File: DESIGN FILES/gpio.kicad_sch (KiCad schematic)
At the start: 12 parts, among them U1 MIMXRT1064CVL5B

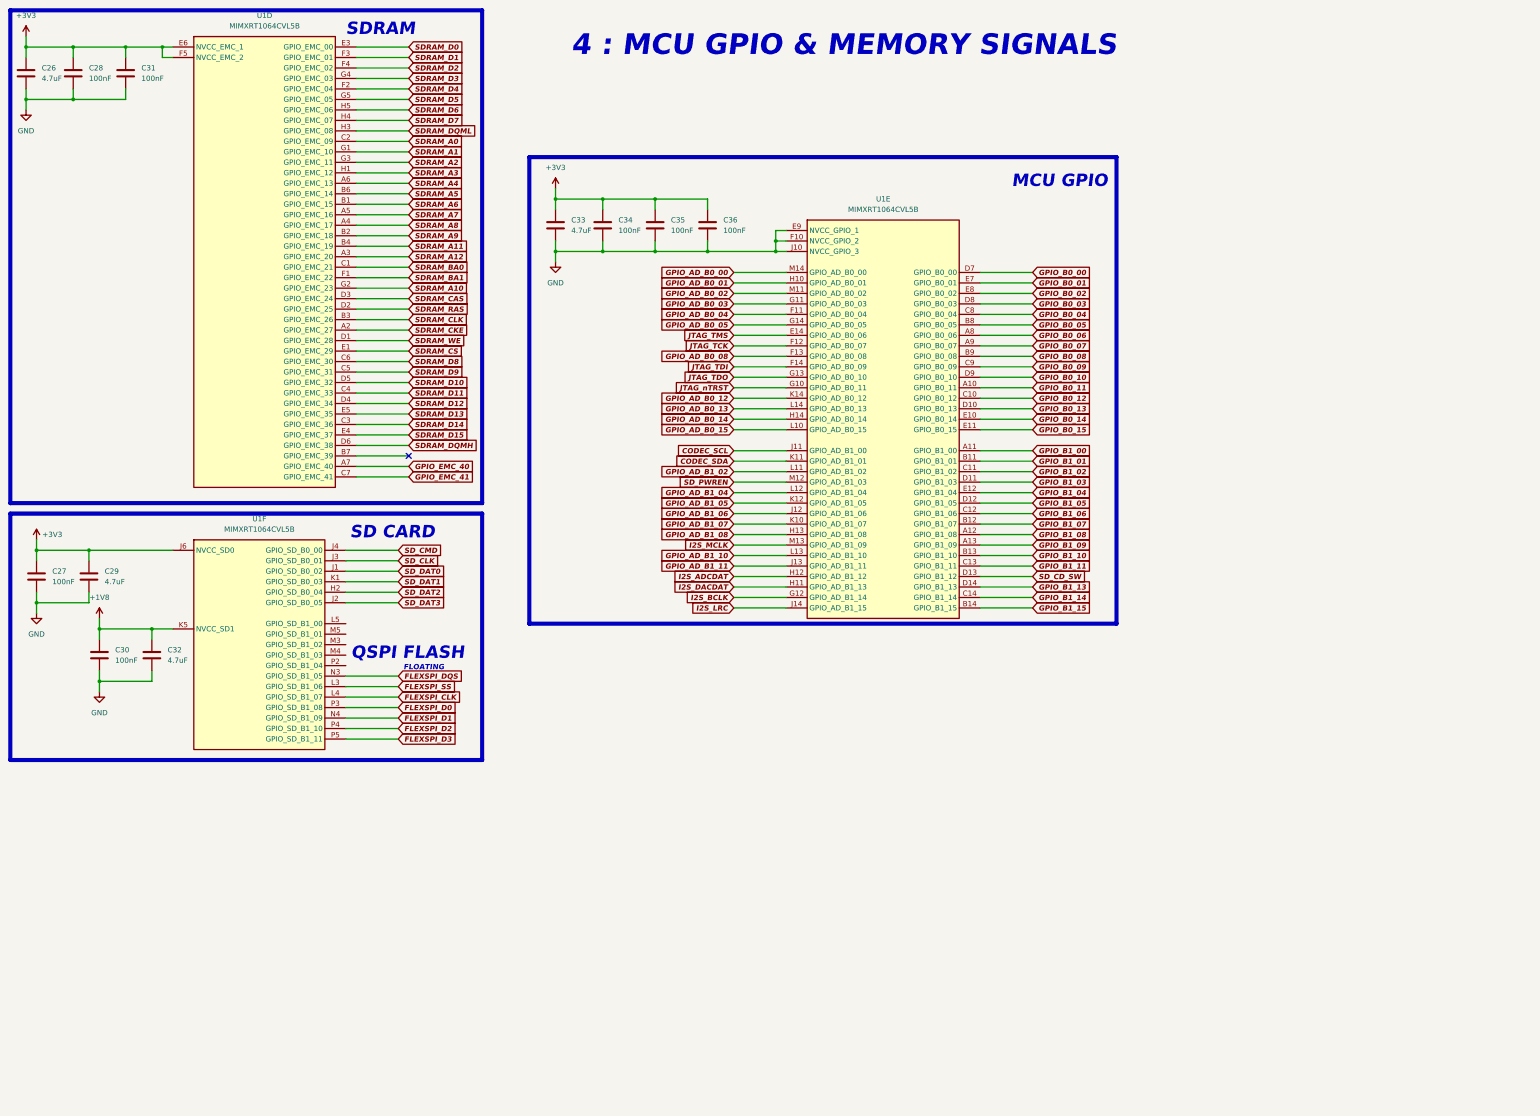
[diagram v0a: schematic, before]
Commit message: schematic edit
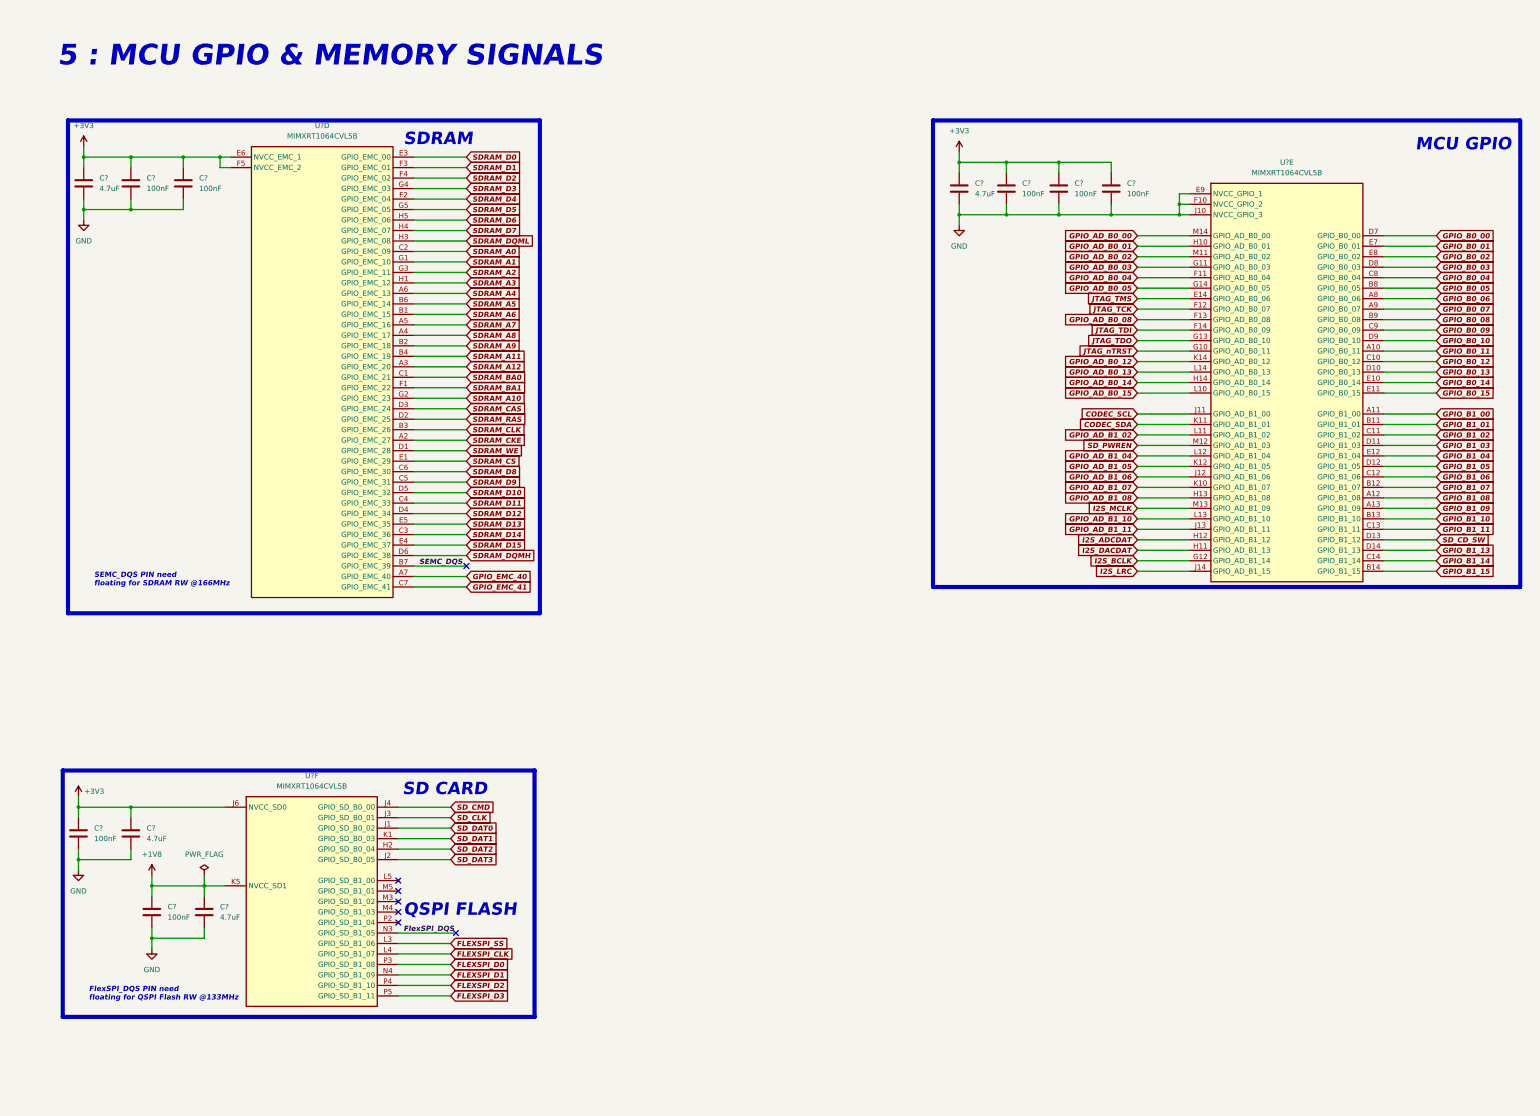
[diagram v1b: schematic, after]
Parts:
- removed C26, C29, C32, C33: 4.7uF, MIMXRT1064 MCU Module:0402_CL05A475MP5NRNC, symbol MIMXRT1064 MCU Module:CL05A475MP5NRNC
- removed C27, C28, C30, C31, C34, C35, C36: 100nF, MIMXRT1064 MCU Module:0402_CL05B104KB54PNC, symbol MIMXRT1064 MCU Module:CL05B104KB54PNC
- removed U1: MIMXRT1064CVL5B, MIMXRT1064 MCU Module:MIMXRT1064CVL5B, symbol MIMXRT1064 MCU Module:MIMXRT1064CVL5B
- added C? (x4): 4.7uF, MIMXRT1064 MCU Module:0402_CL05A475MP5NRNC, symbol MIMXRT1064 MCU Module:CL05A475MP5NRNC
- added C? (x7): 100nF, MIMXRT1064 MCU Module:0402_CL05B104KB54PNC, symbol MIMXRT1064 MCU Module:CL05B104KB54PNC
- added U? (x3): MIMXRT1064CVL5B, MIMXRT1064 MCU Module:MIMXRT1064CVL5B, symbol MIMXRT1064 MCU Module:MIMXRT1064CVL5B
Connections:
- net +1V8: now also C?.1, C?.1, U?.K5 (NVCC_SD1)
- net +3V3: now also C?.1, C?.1, C?.1, C?.1, C?.1, C?.1, C?.1, C?.1, C?.1, U?.E6 (NVCC_EMC_1), U?.F5 (NVCC_EMC_2), U?.J6 (NVCC_SD0)
- net CODEC_SCL: now also U?.J11 (GPIO_AD_B1_00)
- net CODEC_SDA: now also U?.K11 (GPIO_AD_B1_01)
- net FLEXSPI_CLK: now also U?.L4 (GPIO_SD_B1_07)
- net FLEXSPI_D0: now also U?.P3 (GPIO_SD_B1_08)
- net FLEXSPI_D1: now also U?.N4 (GPIO_SD_B1_09)
- net FLEXSPI_D2: now also U?.P4 (GPIO_SD_B1_10)
- net FLEXSPI_D3: now also U?.P5 (GPIO_SD_B1_11)
- net FLEXSPI_SS: now also U?.L3 (GPIO_SD_B1_06)
- net GND: now also C?.2, C?.2, C?.2, C?.2, C?.2, C?.2, C?.2, C?.2, C?.2, C?.2, C?.2, U?.E9 (NVCC_GPIO_1), U?.F10 (NVCC_GPIO_2), U?.J10 (NVCC_GPIO_3)
- net GPIO_AD_B0_00: now also U?.M14 (GPIO_AD_B0_00)
- net GPIO_AD_B0_01: now also U?.H10 (GPIO_AD_B0_01)
- net GPIO_AD_B0_02: now also U?.M11 (GPIO_AD_B0_02)
- net GPIO_AD_B0_03: now also U?.G11 (GPIO_AD_B0_03)
- net GPIO_AD_B0_04: now also U?.F11 (GPIO_AD_B0_04)
- net GPIO_AD_B0_05: now also U?.G14 (GPIO_AD_B0_05)
- net GPIO_AD_B0_08: now also U?.F13 (GPIO_AD_B0_08)
- net GPIO_AD_B0_12: now also U?.K14 (GPIO_AD_B0_12)
- net GPIO_AD_B0_13: now also U?.L14 (GPIO_AD_B0_13)
- net GPIO_AD_B0_14: now also U?.H14 (GPIO_AD_B0_14)
- net GPIO_AD_B0_15: now also U?.L10 (GPIO_AD_B0_15)
- net GPIO_AD_B1_02: now also U?.L11 (GPIO_AD_B1_02)
- net GPIO_AD_B1_04: now also U?.L12 (GPIO_AD_B1_04)
- net GPIO_AD_B1_05: now also U?.K12 (GPIO_AD_B1_05)
- net GPIO_AD_B1_06: now also U?.J12 (GPIO_AD_B1_06)
- net GPIO_AD_B1_07: now also U?.K10 (GPIO_AD_B1_07)
- net GPIO_AD_B1_08: now also U?.H13 (GPIO_AD_B1_08)
- net GPIO_AD_B1_10: now also U?.L13 (GPIO_AD_B1_10)
- net GPIO_AD_B1_11: now also U?.J13 (GPIO_AD_B1_11)
- net GPIO_B0_00: now also U?.D7 (GPIO_B0_00)
- net GPIO_B0_01: now also U?.E7 (GPIO_B0_01)
- net GPIO_B0_02: now also U?.E8 (GPIO_B0_02)
- net GPIO_B0_03: now also U?.D8 (GPIO_B0_03)
- net GPIO_B0_04: now also U?.C8 (GPIO_B0_04)
- net GPIO_B0_05: now also U?.B8 (GPIO_B0_05)
- net GPIO_B0_06: now also U?.A8 (GPIO_B0_06)
- net GPIO_B0_07: now also U?.A9 (GPIO_B0_07)
- net GPIO_B0_08: now also U?.B9 (GPIO_B0_08)
- net GPIO_B0_09: now also U?.C9 (GPIO_B0_09)
- net GPIO_B0_10: now also U?.D9 (GPIO_B0_10)
- net GPIO_B0_11: now also U?.A10 (GPIO_B0_11)
- net GPIO_B0_12: now also U?.C10 (GPIO_B0_12)
- net GPIO_B0_13: now also U?.D10 (GPIO_B0_13)
- net GPIO_B0_14: now also U?.E10 (GPIO_B0_14)
- net GPIO_B0_15: now also U?.E11 (GPIO_B0_15)
- net GPIO_B1_00: now also U?.A11 (GPIO_B1_00)
- net GPIO_B1_01: now also U?.B11 (GPIO_B1_01)
- net GPIO_B1_02: now also U?.C11 (GPIO_B1_02)
- net GPIO_B1_03: now also U?.D11 (GPIO_B1_03)
- net GPIO_B1_04: now also U?.E12 (GPIO_B1_04)
- net GPIO_B1_05: now also U?.D12 (GPIO_B1_05)
- net GPIO_B1_06: now also U?.C12 (GPIO_B1_06)
- net GPIO_B1_07: now also U?.B12 (GPIO_B1_07)
- net GPIO_B1_08: now also U?.A12 (GPIO_B1_08)
- net GPIO_B1_09: now also U?.A13 (GPIO_B1_09)
- net GPIO_B1_10: now also U?.B13 (GPIO_B1_10)
- net GPIO_B1_11: now also U?.C13 (GPIO_B1_11)
- net GPIO_B1_13: now also U?.D14 (GPIO_B1_13)
- net GPIO_B1_14: now also U?.C14 (GPIO_B1_14)
- net GPIO_B1_15: now also U?.B14 (GPIO_B1_15)
- net GPIO_EMC_40: now also U?.A7 (GPIO_EMC_40)
- net GPIO_EMC_41: now also U?.C7 (GPIO_EMC_41)
- net I2S_ADCDAT: now also U?.H12 (GPIO_AD_B1_12)
- net I2S_BCLK: now also U?.G12 (GPIO_AD_B1_14)
- net I2S_DACDAT: now also U?.H11 (GPIO_AD_B1_13)
- net I2S_LRC: now also U?.J14 (GPIO_AD_B1_15)
- net I2S_MCLK: now also U?.M13 (GPIO_AD_B1_09)
- net JTAG_TCK: now also U?.F12 (GPIO_AD_B0_07)
- net JTAG_TDI: now also U?.F14 (GPIO_AD_B0_09)
- net JTAG_TDO: now also U?.G13 (GPIO_AD_B0_10)
- net JTAG_TMS: now also U?.E14 (GPIO_AD_B0_06)
- net JTAG_nTRST: now also U?.G10 (GPIO_AD_B0_11)
- net SDRAM_A0: now also U?.C2 (GPIO_EMC_09)
- net SDRAM_A1: now also U?.G1 (GPIO_EMC_10)
- net SDRAM_A10: now also U?.G2 (GPIO_EMC_23)
- net SDRAM_A11: now also U?.B4 (GPIO_EMC_19)
- net SDRAM_A12: now also U?.A3 (GPIO_EMC_20)
- net SDRAM_A2: now also U?.G3 (GPIO_EMC_11)
- net SDRAM_A3: now also U?.H1 (GPIO_EMC_12)
- net SDRAM_A4: now also U?.A6 (GPIO_EMC_13)
- net SDRAM_A5: now also U?.B6 (GPIO_EMC_14)
- net SDRAM_A6: now also U?.B1 (GPIO_EMC_15)
- net SDRAM_A7: now also U?.A5 (GPIO_EMC_16)
- net SDRAM_A8: now also U?.A4 (GPIO_EMC_17)
- net SDRAM_A9: now also U?.B2 (GPIO_EMC_18)
- net SDRAM_BA0: now also U?.C1 (GPIO_EMC_21)
- net SDRAM_BA1: now also U?.F1 (GPIO_EMC_22)
- net SDRAM_CAS: now also U?.D3 (GPIO_EMC_24)
- net SDRAM_CKE: now also U?.A2 (GPIO_EMC_27)
- net SDRAM_CLK: now also U?.B3 (GPIO_EMC_26)
- net SDRAM_CS: now also U?.E1 (GPIO_EMC_29)
- net SDRAM_D0: now also U?.E3 (GPIO_EMC_00)
- net SDRAM_D1: now also U?.F3 (GPIO_EMC_01)
- net SDRAM_D10: now also U?.D5 (GPIO_EMC_32)
- net SDRAM_D11: now also U?.C4 (GPIO_EMC_33)
- net SDRAM_D12: now also U?.D4 (GPIO_EMC_34)
- net SDRAM_D13: now also U?.E5 (GPIO_EMC_35)
- net SDRAM_D14: now also U?.C3 (GPIO_EMC_36)
- net SDRAM_D15: now also U?.E4 (GPIO_EMC_37)
- net SDRAM_D2: now also U?.F4 (GPIO_EMC_02)
- net SDRAM_D3: now also U?.G4 (GPIO_EMC_03)
- net SDRAM_D4: now also U?.F2 (GPIO_EMC_04)
- net SDRAM_D5: now also U?.G5 (GPIO_EMC_05)
- net SDRAM_D6: now also U?.H5 (GPIO_EMC_06)
- net SDRAM_D7: now also U?.H4 (GPIO_EMC_07)
- net SDRAM_D8: now also U?.C6 (GPIO_EMC_30)
- net SDRAM_D9: now also U?.C5 (GPIO_EMC_31)
- net SDRAM_DQMH: now also U?.D6 (GPIO_EMC_38)
- net SDRAM_DQML: now also U?.H3 (GPIO_EMC_08)
- net SDRAM_RAS: now also U?.D2 (GPIO_EMC_25)
- net SDRAM_WE: now also U?.D1 (GPIO_EMC_28)
- net SD_CD_SW: now also U?.D13 (GPIO_B1_12)
- net SD_CLK: now also U?.J3 (GPIO_SD_B0_01)
- net SD_CMD: now also U?.J4 (GPIO_SD_B0_00)
- net SD_DAT0: now also U?.J1 (GPIO_SD_B0_02)
- net SD_DAT1: now also U?.K1 (GPIO_SD_B0_03)
- net SD_DAT2: now also U?.H2 (GPIO_SD_B0_04)
- net SD_DAT3: now also U?.J2 (GPIO_SD_B0_05)
- net SD_PWREN: now also U?.M12 (GPIO_AD_B1_03)
- new net FlexSPI_DQS: U?.N3 (GPIO_SD_B1_05)
- new net SEMC_DQS: U?.B7 (GPIO_EMC_39)
- no-connect marks 1 -> 7
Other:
- note added: "5 : MCU GPIO & MEMORY SIGNALS"
- note added: "FlexSPI_DQS PIN need floating for QSPI Flash RW @133MHz"
- note added: "SEMC_DQS PIN need floating for SDRAM RW @166MHz"
- note removed: "4 : MCU GPIO & MEMORY SIGNALS"
- note removed: "FLOATING"
- title: MCU GPIO & Memory signals -> Memory & USB

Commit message: schematic changes
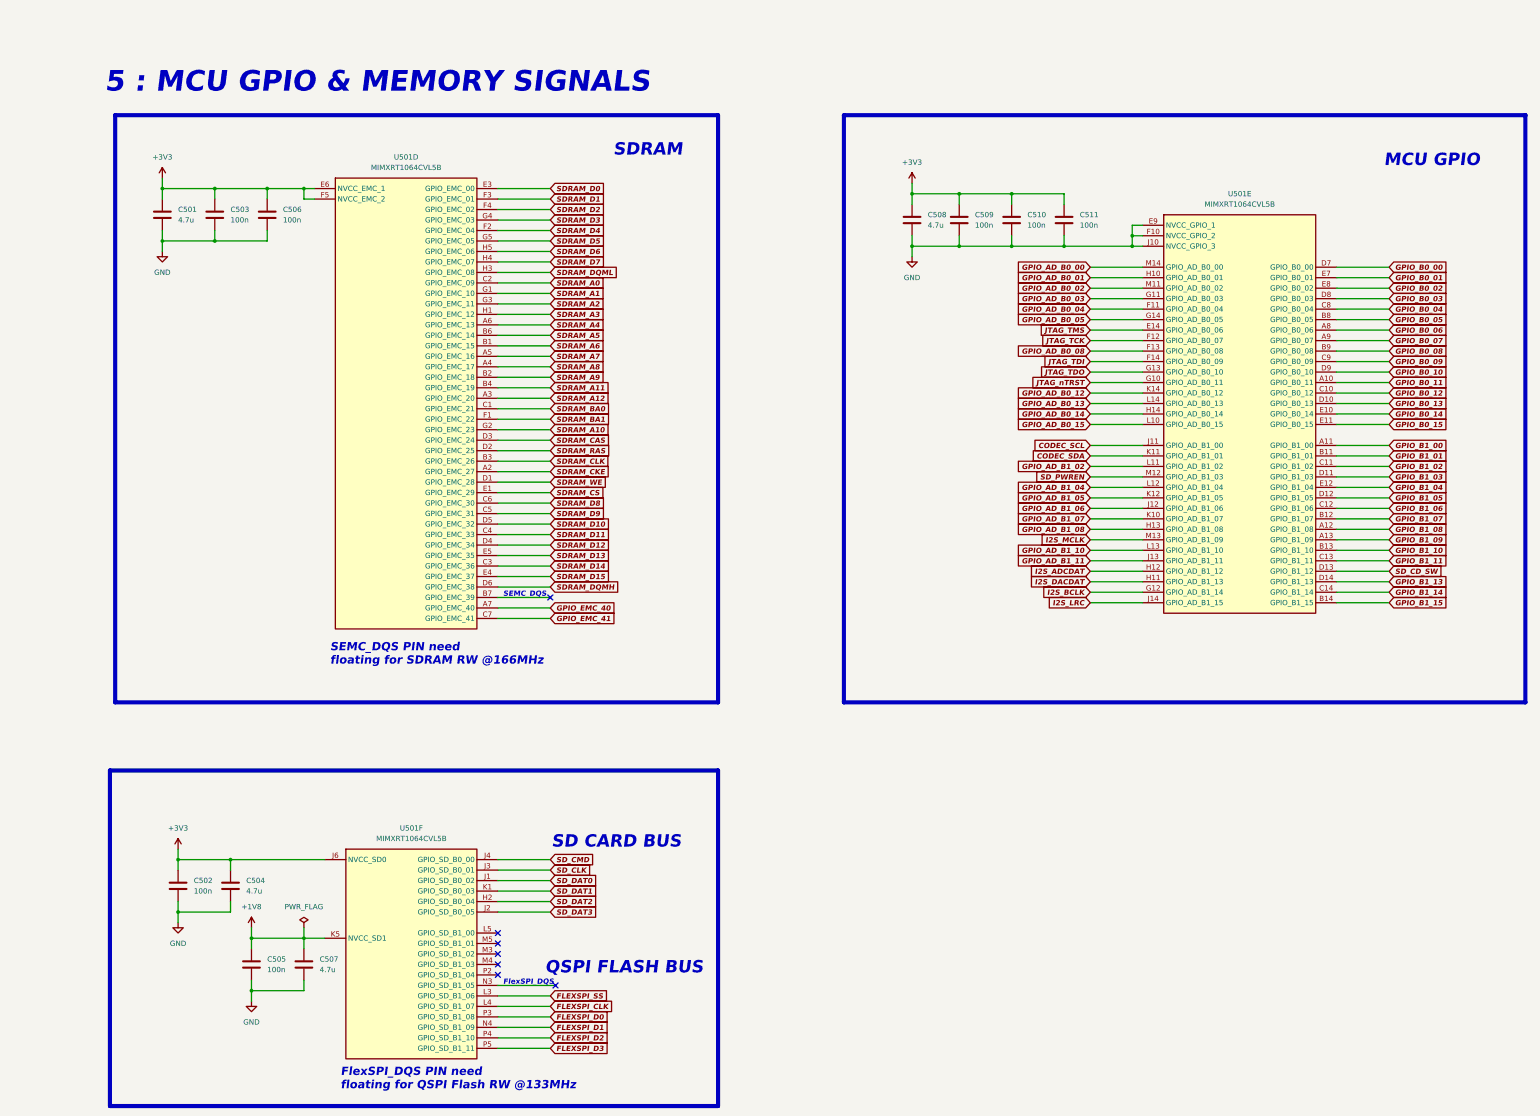
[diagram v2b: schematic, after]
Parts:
- C501, C504, C507, C508: renamed from C?; value 4.7uF -> 4.7u
- C502, C503, C505, C506, C509, C510, C511: renamed from C?; value 100nF -> 100n
- gave numbers to parts that had none: 1
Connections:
- net FlexSPI_DQS: no longer names the net of U501.N3 (GPIO_SD_B1_05)
- net SEMC_DQS: no longer names the net of U501.B7 (GPIO_EMC_39)
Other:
- note added: "FlexSPI_DQS"
- note added: "QSPI FLASH BUS"
- note added: "SD CARD BUS"
- note added: "SEMC_DQS"
- note removed: "QSPI FLASH"
- note removed: "SD CARD"
- moved on the sheet: C501, C502, C503, C504, C505, C506, C507, C508, C509, C510, C511, U501D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
